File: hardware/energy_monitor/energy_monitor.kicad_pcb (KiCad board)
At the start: 4 copper layers, 102.8 x 86.9 mm, 137 parts, among them J1 Screw_Terminal_01x03, J2 SJ1-3533NG, J3 SJ1-3533NG, J4 SJ1-3533NG, J5 SJ1-3533NG, J6 SJ1-3533NG, J7 SJ1-3533NG, J8 USB_OTG, Q1 MMBT2222, Q2 MMBT2222, U1 RAC04, U2 TPS730, U3 TPS723, U4 ADS131E08, U5 AP2112, U6 ESP-WROOM-32U, U7 CP2104

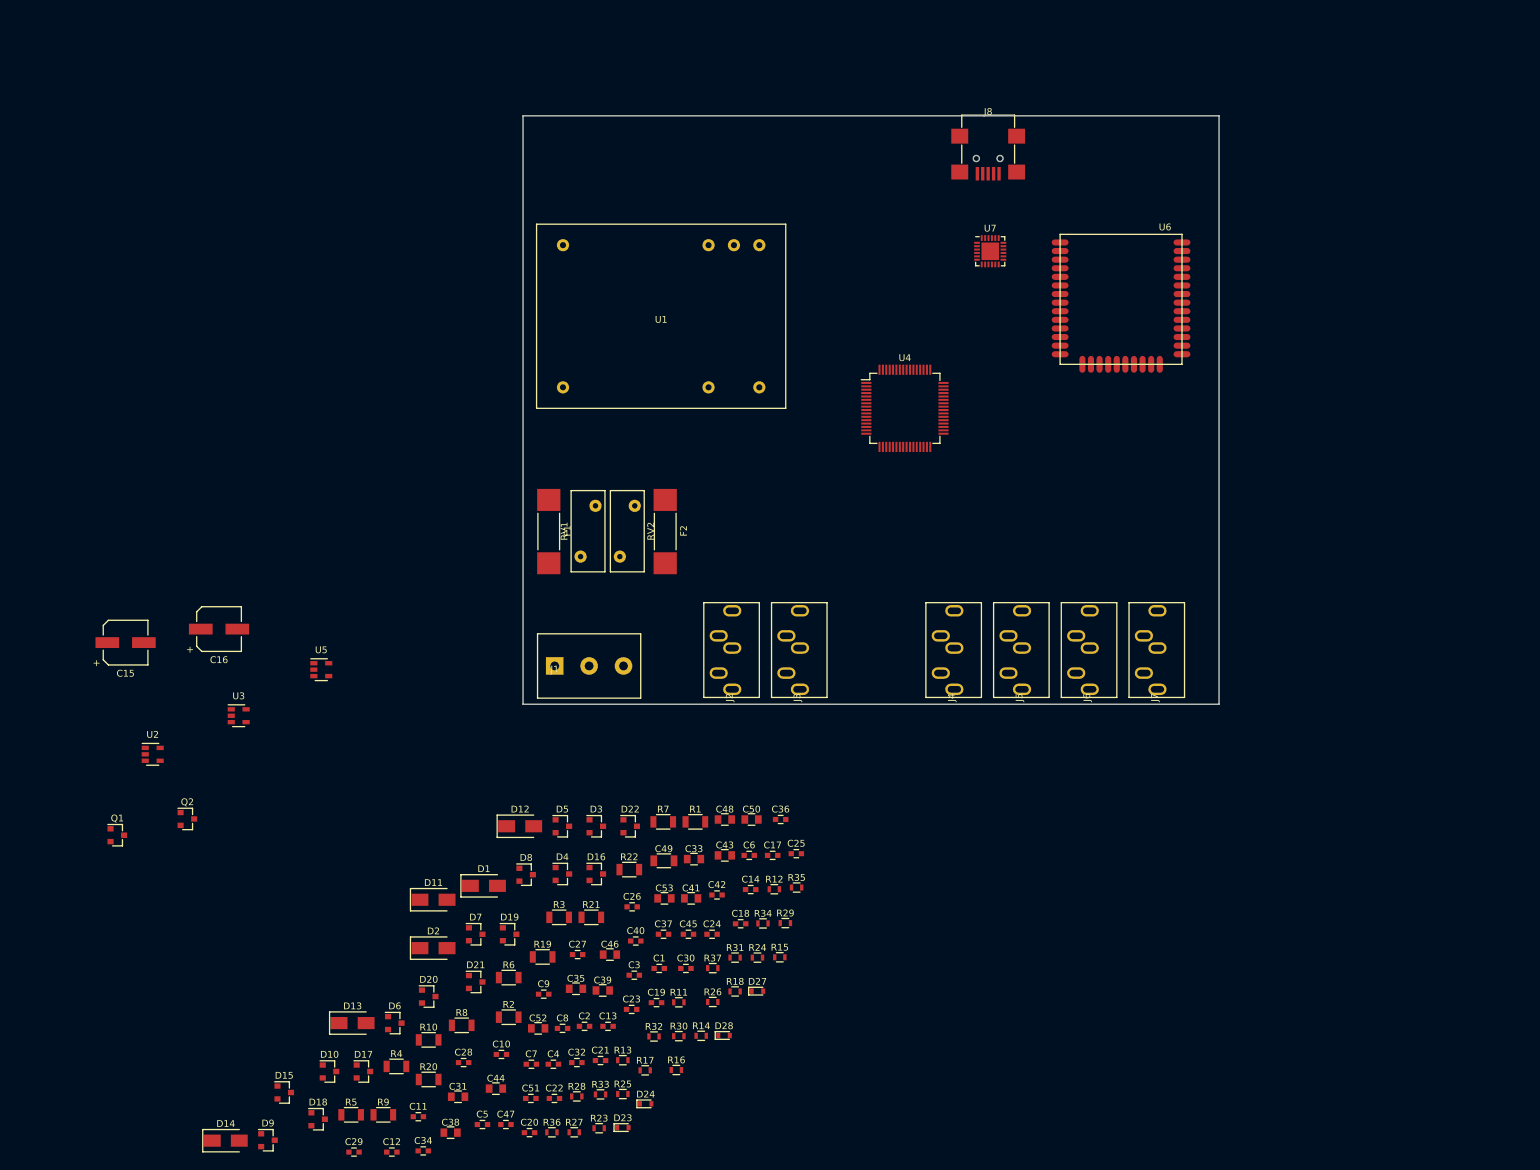
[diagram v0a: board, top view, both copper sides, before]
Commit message: Working on layout
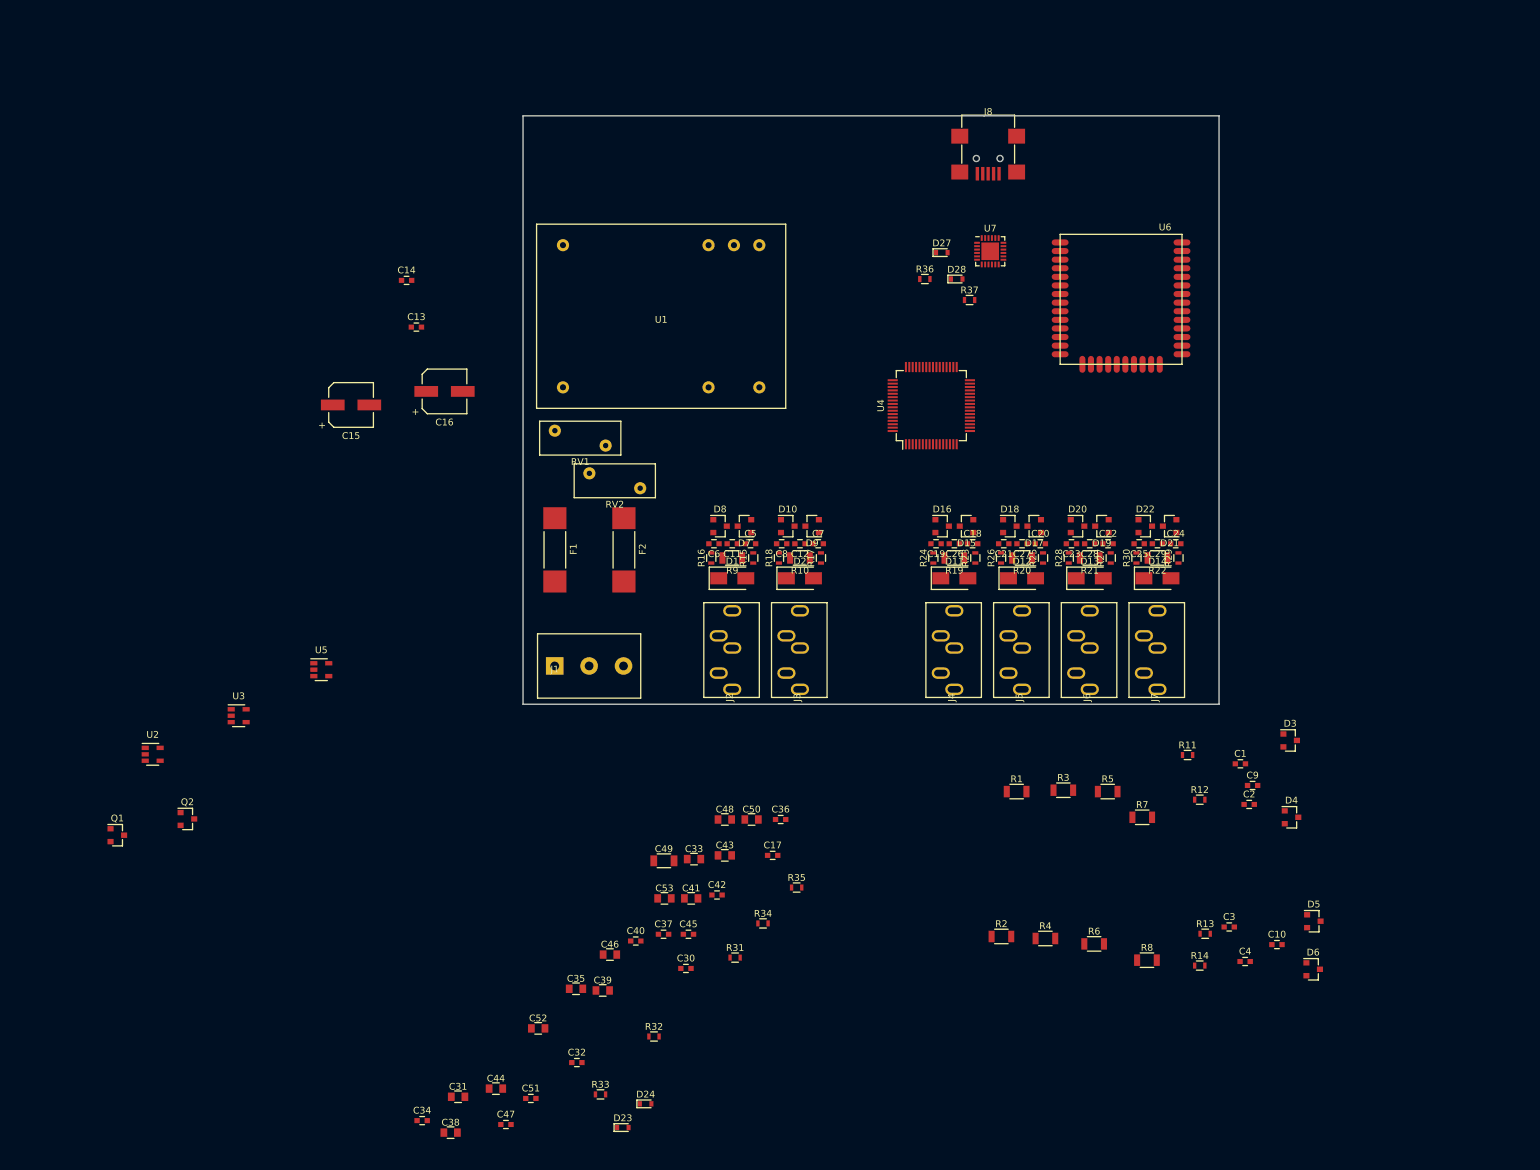
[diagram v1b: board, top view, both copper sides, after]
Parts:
- C31, C38: value 2.2u -> 10u
- moved D14 160.7 mm to (183.7, 101.4)
- moved C29 148.8 mm to (183.7, 96.3), turned to 180 degrees
- moved R36 137.5 mm to (149.3, 57.2)
- moved D6 135.9 mm to (206.7, 159.2)
- moved D18 134.6 mm to (161.9, 93.7)
- moved D15 131.0 mm to (155.5, 93.7), turned to 180 degrees
- moved D17 127.7 mm to (165.5, 93.7), turned to 180 degrees
- moved D13 127.2 mm to (173.7, 101.4)
- moved D21 122.6 mm to (185.5, 93.7), turned to 180 degrees
- moved R5 121.5 mm to (176.3, 132.9)
- moved D9 121.2 mm to (132.7, 93.7), turned to 180 degrees
- moved C28 120.1 mm to (173.7, 96.3), turned to 180 degrees
- moved D20 118.4 mm to (171.9, 93.7)
- moved D28 116.9 mm to (154.1, 57.2)
- moved R20 116.7 mm to (163.7, 98.4), turned to 180 degrees
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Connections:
- net GND renamed GNDA
- U4 pad 1: /I6_N -> /L1_N
- U4 pad 10: /I2_P -> /I3_P
- U4 pad 11: /I1_N -> /I4_N
- U4 pad 12: /I1_P -> /I4_P
- U4 pad 13: /L2_N -> /I5_N
- U4 pad 14: /L2_P -> /I5_P
- U4 pad 15: /L1_N -> /I6_N
- U4 pad 16: /L1_P -> /I6_P
- U4 pad 2: /I6_P -> /L1_P
- U4 pad 3: /I5_N -> /L2_N
- U4 pad 4: /I5_P -> /L2_P
- U4 pad 5: /I4_N -> /I1_N
- U4 pad 6: /I4_P -> /I1_P
- U4 pad 7: /I3_N -> /I2_N
- U4 pad 8: /I3_P -> /I2_P
- U4 pad 9: /I2_N -> /I3_N

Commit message: Working on layout
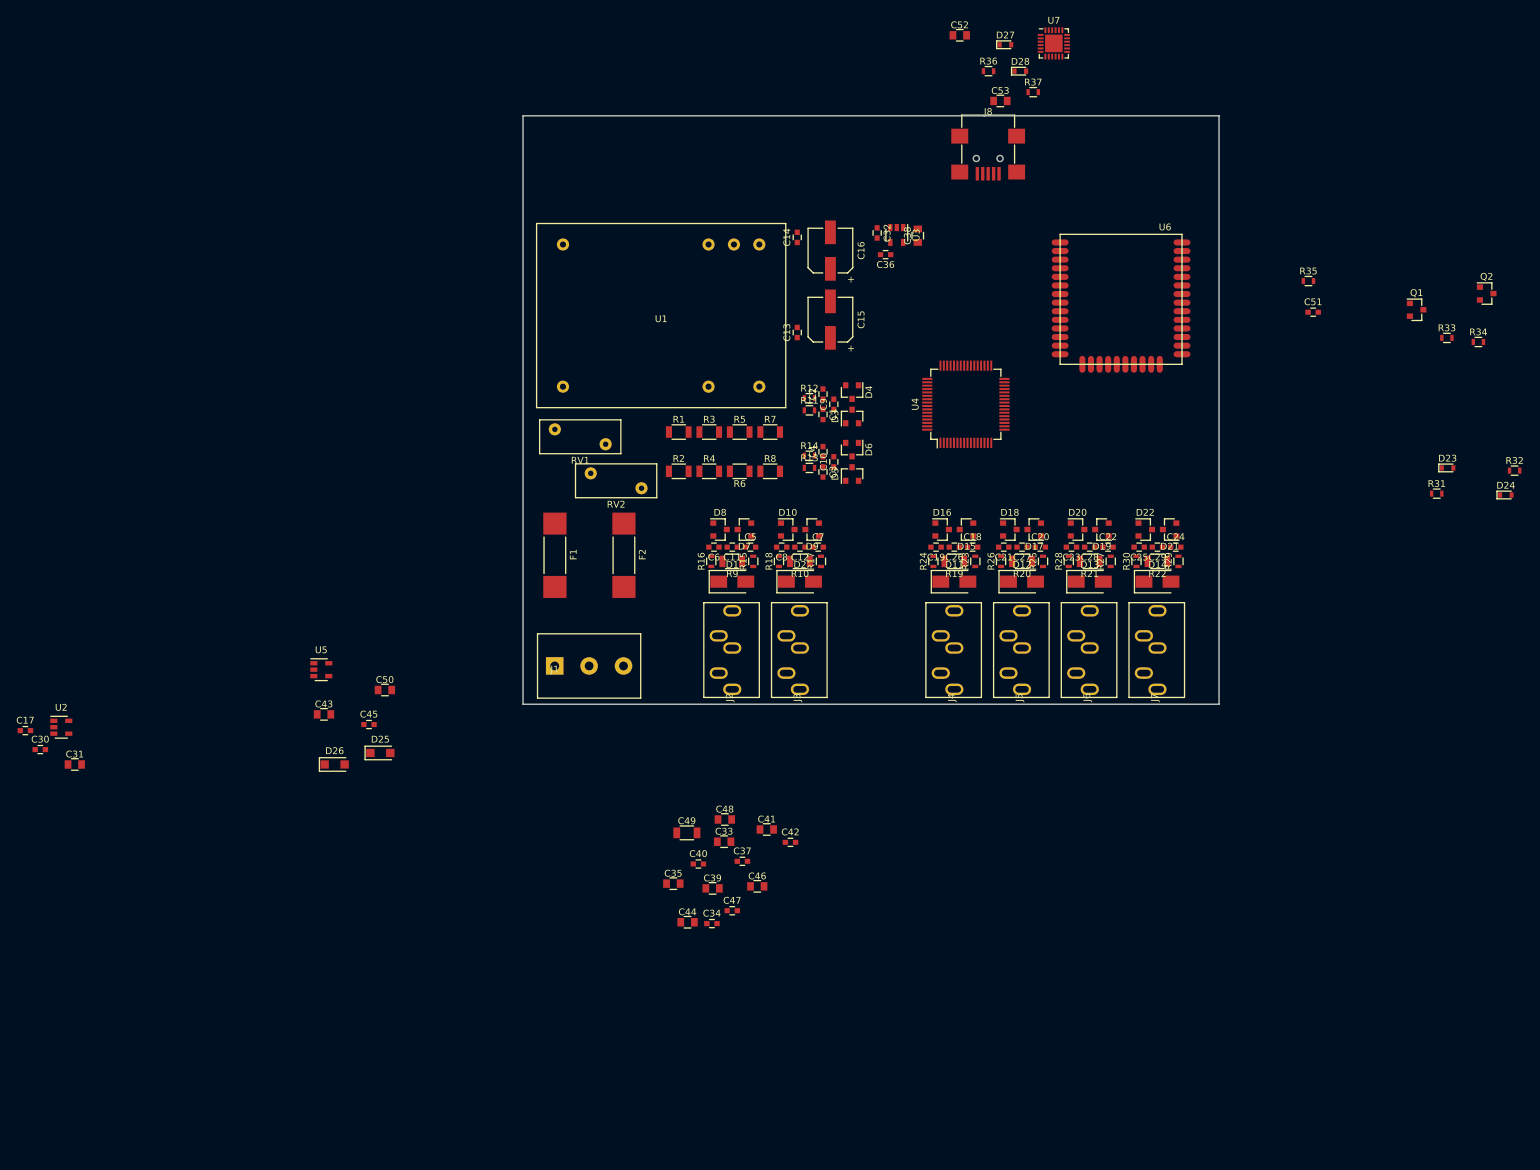
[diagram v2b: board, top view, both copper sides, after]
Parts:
- added D25: MBR120, footprint:SOD-123FL, F.Cu at (68.9, 127.2)
- added D26: MBR120, footprint:SOD-123FL, F.Cu at (62.2, 128.9)
- moved Q1 207.0 mm to (222.0, 61.7)
- moved Q2 207.0 mm to (232.3, 59.3)
- moved R33 167.7 mm to (226.4, 65.9)
- moved C51 163.8 mm to (206.7, 62.1)
- moved C52 159.3 mm to (154.5, 21.2)
- moved D23 156.0 mm to (226.6, 85.1)
- moved D24 155.6 mm to (235.2, 89.1)
- moved R32 152.1 mm to (236.4, 85.5)
- moved C38 149.4 mm to (148.3, 50.8), turned to 90 degrees
- moved R34 136.2 mm to (231.1, 66.5)
- moved C32 130.3 mm to (142.3, 50.4), turned to 270 degrees
- moved C53 127.8 mm to (160.5, 30.9)
- moved R31 124.2 mm to (224.9, 88.9)
- moved U3 120.4 mm to (145.2, 50.7), turned to 270 degrees
- moved R35 117.2 mm to (206.0, 57.5)
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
